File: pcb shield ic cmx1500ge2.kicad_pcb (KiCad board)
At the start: 2 copper layers, 68.6 x 53.3 mm, 14 parts, among them P1 Power, P2 Analog, P3 Digital, P4 Digital, P5 CONN_01X01, P6 CONN_01X01, P7 CONN_01X01, P8 CONN_01X01

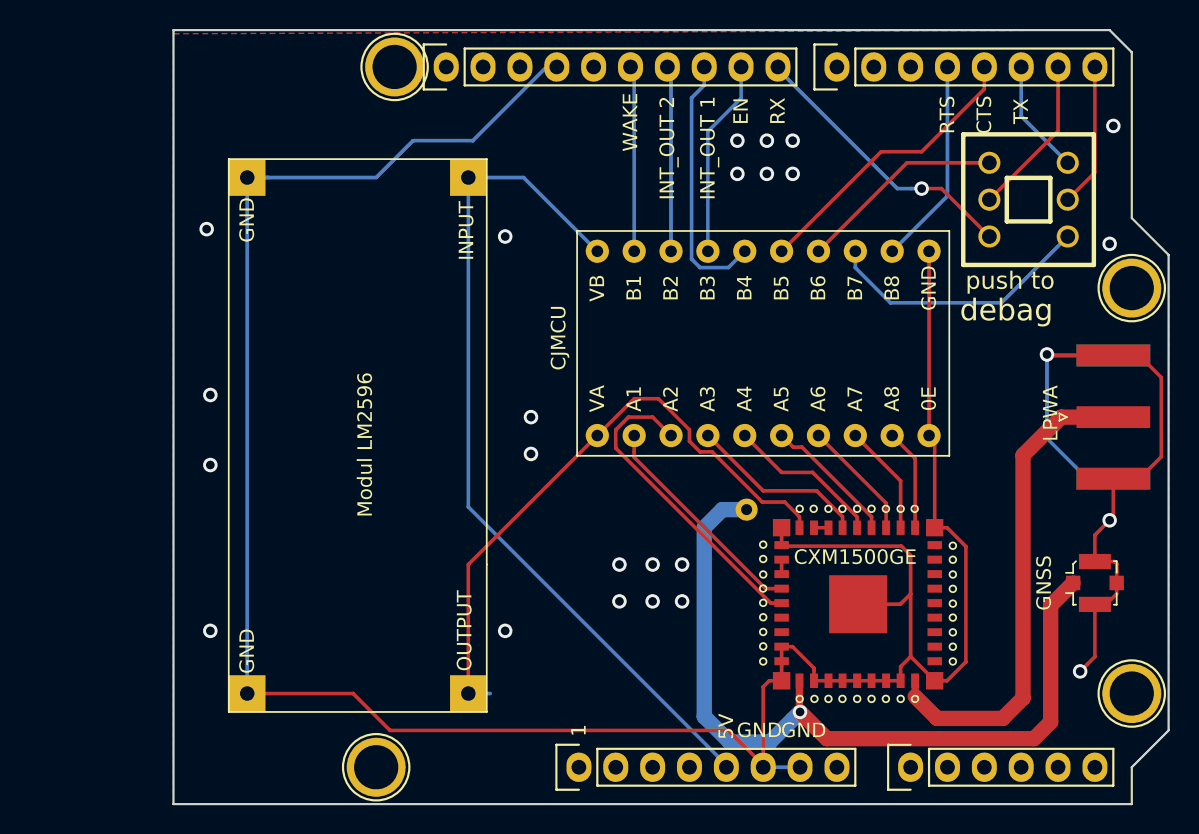
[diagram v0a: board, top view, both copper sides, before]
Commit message: initial commit
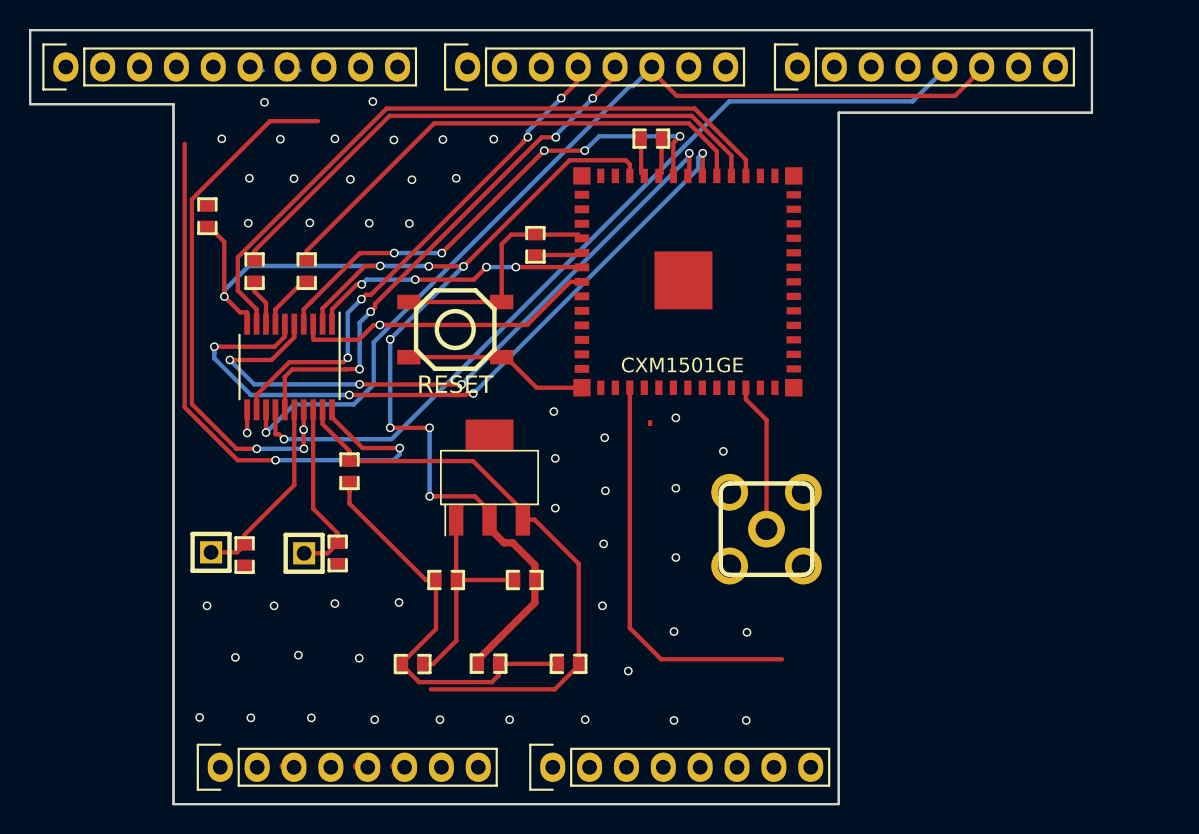
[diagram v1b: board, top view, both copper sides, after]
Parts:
- removed CJMCU: modul_lvl-conveter_cjmcu, modul:modul_lvl_conveter_cjmcu
- removed CXM1500GE: CXM1500GE, modul:CXM1500GE
- removed GNSS: SMA, Connector_Coaxial:U.FL_Molex_MCRF_73412-0110_Vertical
- removed LM2596_1: modul_dc-dc_lm2596, modul:modul_lvl_dc-dc_lm2596
- removed LPWA: SMA, Connector_Coaxial:SMA_Amphenol_132289_EdgeMount
- removed P5, P6, P8: CONN_01X01, Socket_Arduino_Uno:Arduino_1pin
- removed push to: SWITCH-DPDT, Switches:Switch_DPDT_6p_TH
- added C1: 100uF, Capacitors:C_Ceramic_SMD_0603, F.Cu at (132.7, 116.7)
- added C2: 0.1u, Capacitors:C_Ceramic_SMD_0603, F.Cu at (113.3, 85.9)
- added C3: 0.1u, Capacitors:C_Ceramic_SMD_0603, F.Cu at (123.1, 103.4)
- added C4: 100uF, Capacitors:C_Ceramic_SMD_0603, F.Cu at (127.5, 116.7)
- added C5: 10uf, Capacitors:C_Ceramic_SMD_0603, F.Cu at (138.2, 116.7)
- added J1: SMA, Connectors_SMA:SMA_Male_Angled_TH, F.Cu at (151.9, 107.4)
- added J3: Conn_01x01_Male, Headers:Pin_Header_1x01_Male_10mil_Straight_TH, F.Cu at (120.0, 109.1)
- added J4: Conn_01x01_Male, Headers:Pin_Header_1x01_Male_10mil_Straight_TH, F.Cu at (113.6, 109.0)
- added R1: 121, Resistors:R_Chip_SMD_0603, F.Cu at (135.2, 110.9)
- added R2: ?, Resistors:R_Chip_SMD_0603, F.Cu at (129.8, 110.9)
- added R3: RES, Resistors:R_Chip_SMD_0603, F.Cu at (135.9, 87.8)
- added R4: RES, Resistors:R_Chip_SMD_0603, F.Cu at (143.9, 80.5)
- added R5: 10, Resistors:R_Chip_SMD_0603, F.Cu at (116.6, 89.6)
- added R6: 10, Resistors:R_Chip_SMD_0603, F.Cu at (120.2, 89.6)
- added R7: -, Resistors:R_Chip_SMD_0603, F.Cu at (122.3, 109.1)
- added R8: -, Resistors:R_Chip_SMD_0603, F.Cu at (115.9, 109.2)
- added REF**: AP2112, AP2112:AP2112, F.Cu at (143.8, 102.1)
- added RESET: BUTTON, Push_Buttons:Button_4p_W-6.0mm_L-6.0mm_Normal_SMD, F.Cu at (130.4, 93.7)
- added U1: CXM1501GE, modul:_CXM1501GE, F.Cu at (153.7, 98.3)
- added U2: TXS0108EPW, Package_SO:TSSOP-20_4.4x6.5mm_P0.65mm, F.Cu at (119.0, 96.2)
- added U3: LM1117-Adj, smd:TO261AA-LM1117_rev, F.Cu at (132.8, 103.9)
- P2: footprint Socket_Arduino_Uno:Socket_Strip_Arduino_1x06 -> Socket_Arduino_Uno:Socket_Strip_Arduino_1x08
- P7: value CONN_01X01 -> Communication; footprint Socket_Arduino_Uno:Arduino_1pin -> Socket_Arduino_Mega:Socket_Strip_Arduino_1x08
- moved P7 27.8 mm to (154.0, 75.6)
- moved P3 26.2 mm to (103.6, 75.6)
- moved P4 25.5 mm to (131.3, 75.6)
- moved P1 24.7 mm to (114.2, 123.8)
- moved P2 24.7 mm to (137.1, 123.8)
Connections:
- P1 pad 1: Net-(P1-Pad1) -> (no net)
- P1 pad 2: /IOREF -> (no net)
- P1 pad 3: /Reset -> (no net)
- P1 pad 4: +3V3 -> (no net)
- P1 pad 8: /Vin -> (no net)
- P2 pad 1: /A0 -> (no net)
- P2 pad 2: /A1 -> (no net)
- P2 pad 3: /A2 -> (no net)
- P2 pad 4: /A3 -> (no net)
- P2 pad 5: /A4(SDA) -> (no net)
- P2 pad 6: /A5(SCL) -> (no net)
- P3 pad 1: /A5(SCL)_l -> (no net)
- P3 pad 10: /8 -> (no net)
- P3 pad 2: /A4(SDA)_l -> (no net)
- P3 pad 3: /AREF -> (no net)
- P3 pad 5: /13(SCK) -> (no net)
- P3 pad 7: /11(**_MOSI) -> (no net)
- P3 pad 8: /10(**_SS) -> (no net)
- P4 pad 1: /7 -> (no net)
- P4 pad 2: /6(**) -> (no net)
- P4 pad 3: /5(**) -> (no net)
- P4 pad 6: /2 -> /19(Rx1)
- P4 pad 7: /1(Tx) -> (no net)
- P4 pad 8: /0(Rx) -> (no net)
- P7 pad 1: Net-(P7-Pad1) -> (no net)
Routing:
- net GND: track 231.6 -> 44.7 mm, vias 25 -> 46
- net /19(Rx1): track 0.00 -> 65.8 mm, vias 0 -> 1
- net /18(Tx1): track 0.00 -> 58.8 mm, vias 0 -> 1
- net /CTS_IC: track 0.00 -> 50.4 mm, vias 0 -> 4
- net /RTS_IC: track 0.00 -> 47.0 mm
- net /INT_1: track 0.00 -> 46.8 mm, vias 0 -> 4
- net Net-(J1-Pad1): track 55.6 -> 10.3 mm, vias 1 -> 0
- net /+2V: track 42.5 -> 86.7 mm, vias 0 -> 8
- net /TX_IC: track 0.00 -> 40.0 mm
- net /RX_IC: track 0.00 -> 35.1 mm
- net /ENB: track 0.00 -> 34.8 mm, vias 0 -> 5
- net /12(MISO): track 12.8 -> 41.7 mm, vias 0 -> 2
- net /9(**): track 13.6 -> 36.9 mm, vias 0 -> 3
- net Net-(TXS0108E-8_1-Pad3): track 21.8 -> 0.00 mm
- net /INT_2: track 0.00 -> 21.2 mm, vias 0 -> 1
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- removed copper zone on B.Cu, net GND
- removed copper zone on F.Cu, net GND
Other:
- board size 68.6 x 53.3 mm -> 73.2 x 53.3 mm
- net class Default: trace_width 0.25 -> 0.3
- net class power added: clearance 0.2, trace_width 0.5, via_dia 0.6, via_drill 0.4
- net class rf: clearance 0.2 -> 0.3; trace_width 1.05736 -> 1.44459
- net class small added: clearance 0.1, trace_width 0.3, via_dia 0.6, via_drill 0.4
- board text removed: "1"
- board text removed: "debag"
